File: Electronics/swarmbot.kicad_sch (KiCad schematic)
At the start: 6 parts, among them J1 12x2 JST, J2 12x2 JST, J7 8P8C

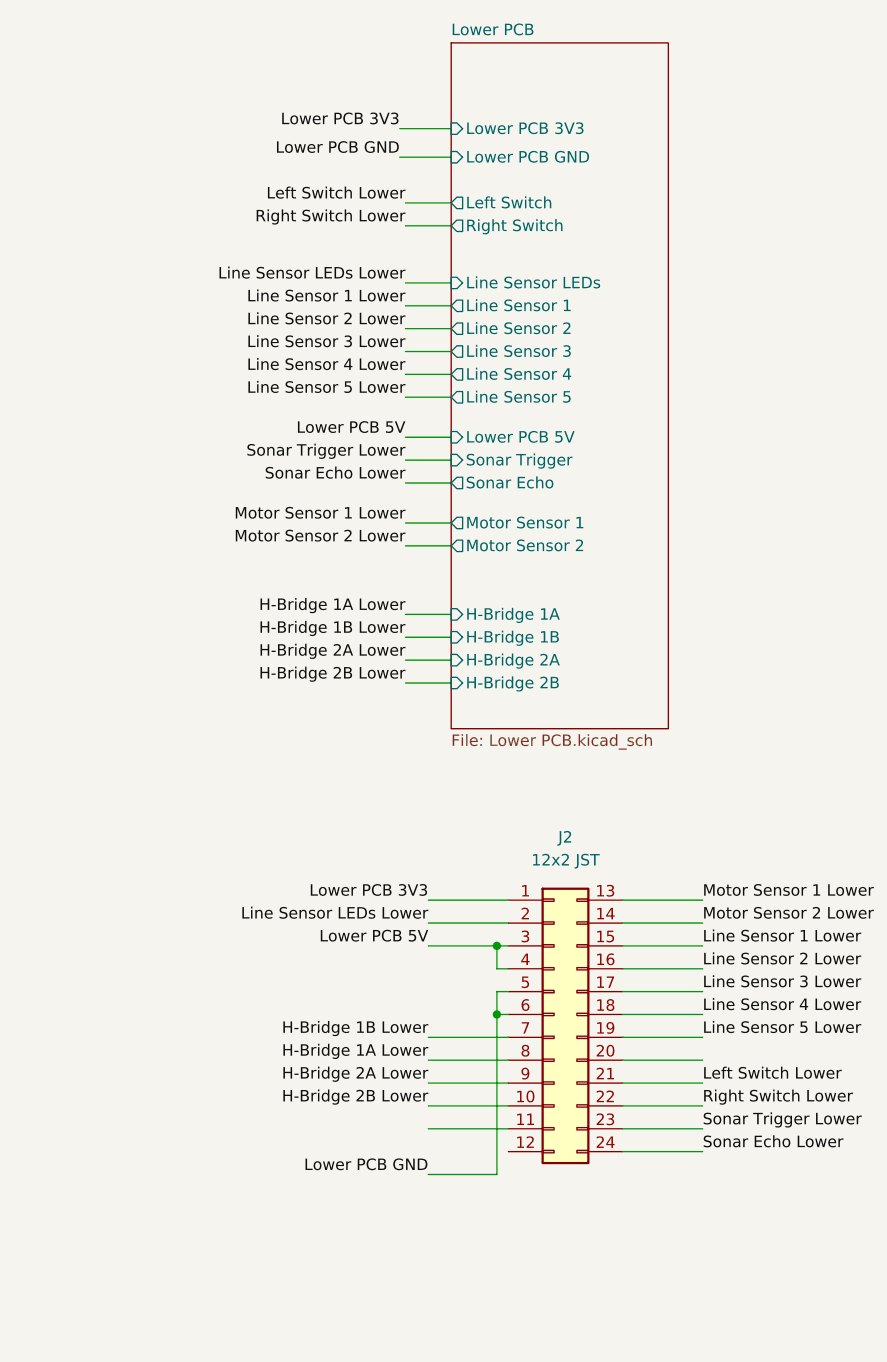
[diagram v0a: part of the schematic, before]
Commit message: made some changes
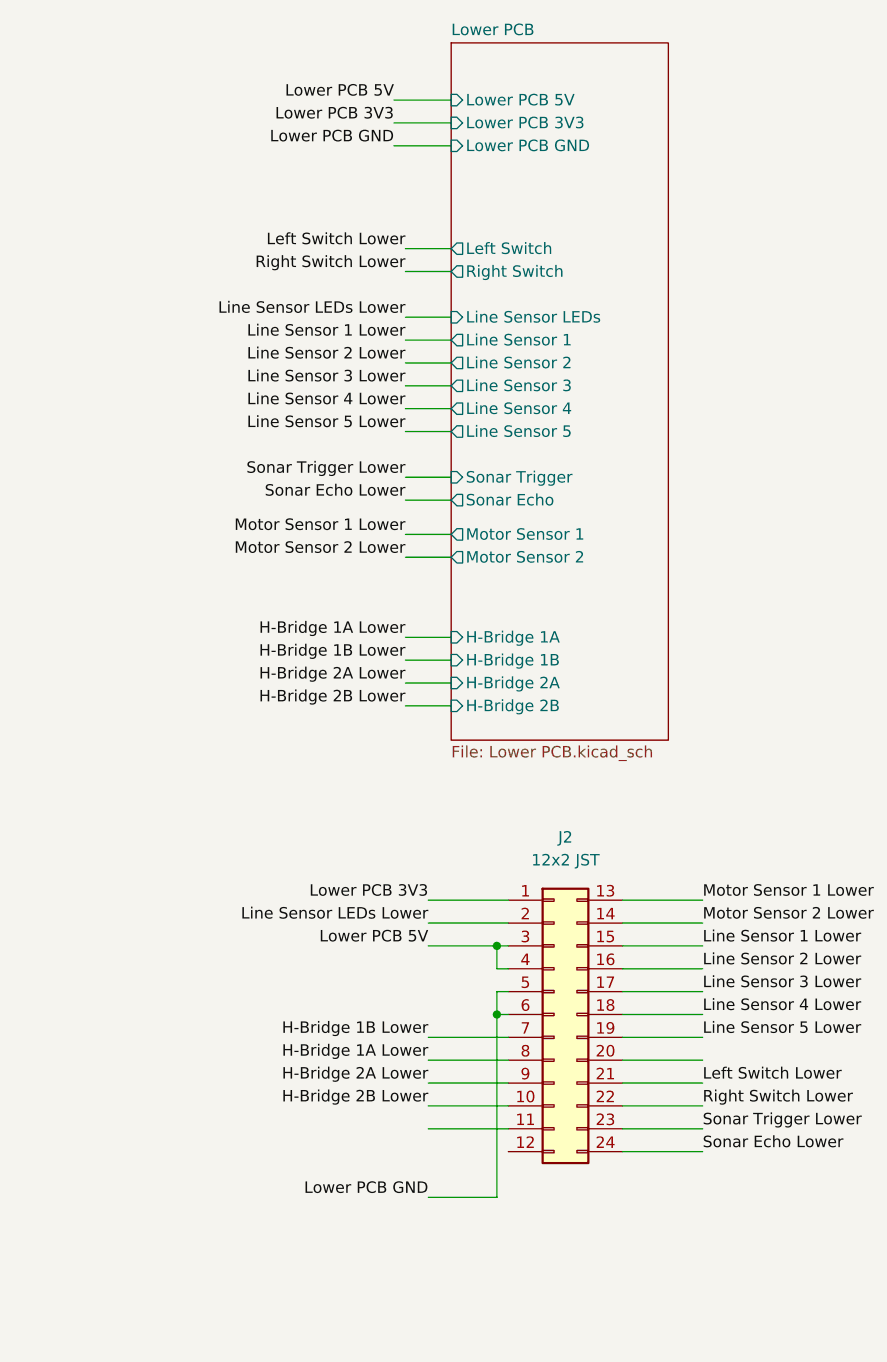
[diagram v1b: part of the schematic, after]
